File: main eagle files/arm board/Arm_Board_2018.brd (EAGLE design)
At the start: 193.8 x 104.4 mm, 152 parts, among them Q1 Q_IRF7437SMD, U1 TIVA-1294, U4 ACS722, U5 ACS722, U6 ACS722, U7 ACS722, U8 ACS722, U9 ACS722

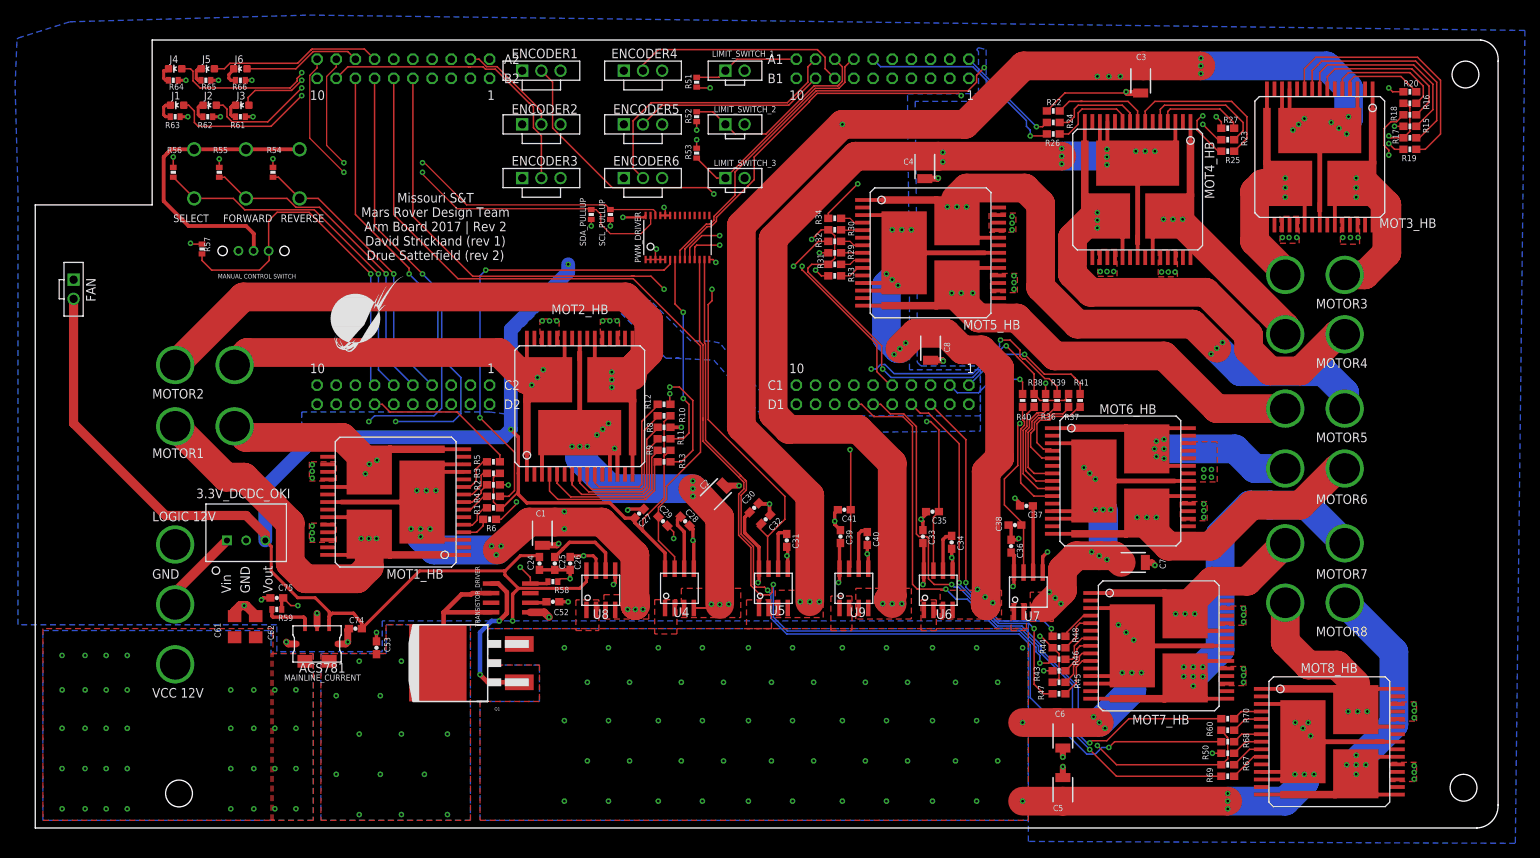
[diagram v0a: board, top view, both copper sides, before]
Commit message: added more polygons
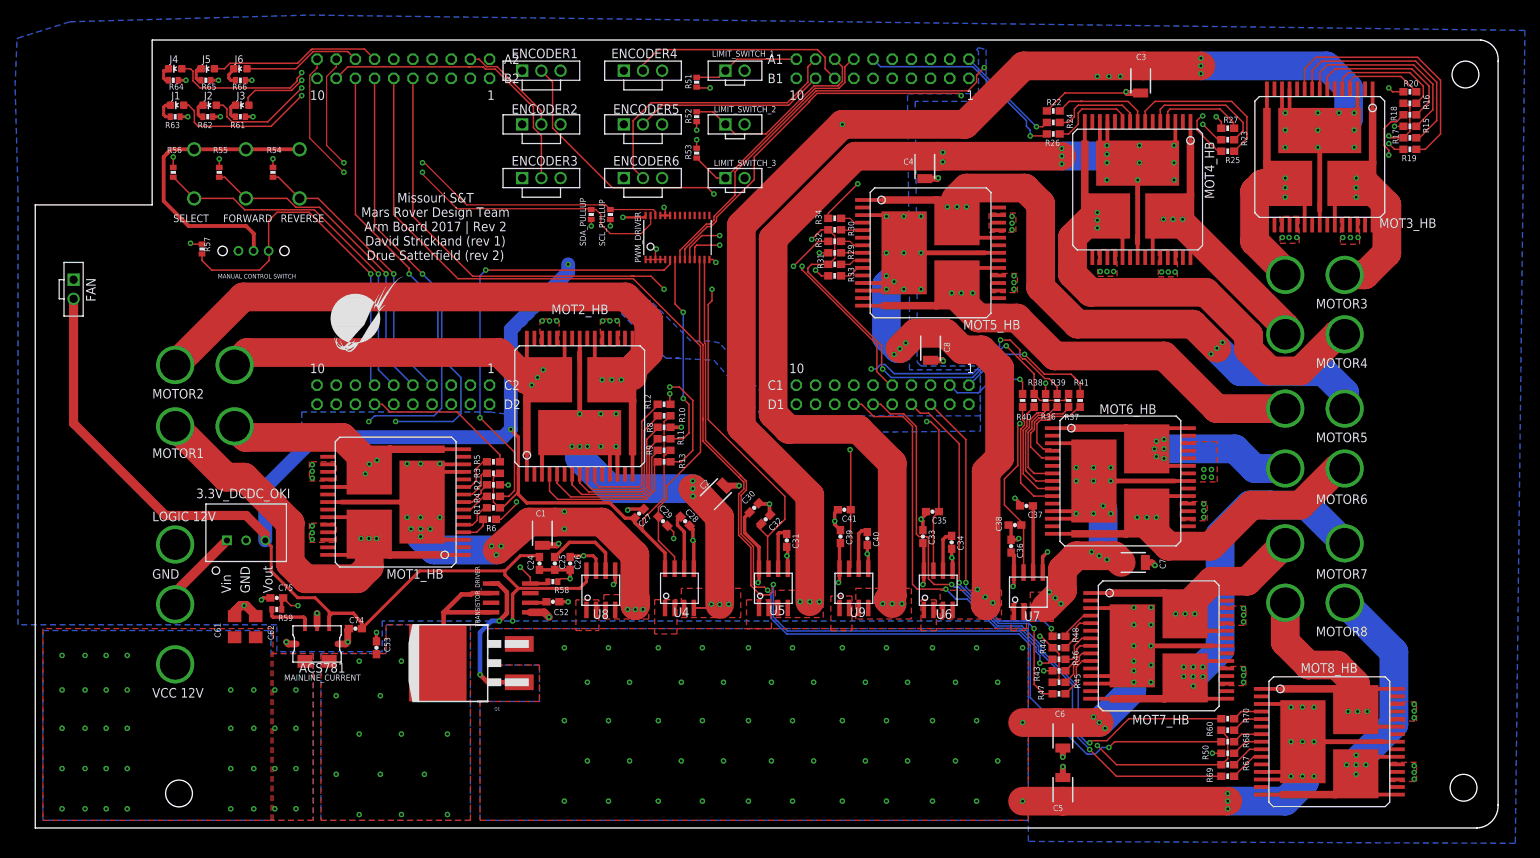
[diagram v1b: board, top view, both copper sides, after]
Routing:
- net MOTOR4_POWER: track 296.1 -> 308.0 mm, vias 14 -> 18
- net MOTOR3_POWER: track 374.3 -> 385.0 mm, vias 17 -> 20
- net MOTOR6_POWER: track 96.2 -> 89.4 mm, vias 12 -> 15
- net MOTOR2_POWER: track 135.4 -> 139.5 mm, vias 13 -> 14
- net MOTOR5_POWER: track 180.4 -> 177.2 mm, vias 12 -> 17
- net MOTOR1_POWER: track 146.1 -> 148.6 mm, vias 15 -> 18
- net 12VMOTOR_POWER: track 242.6 -> 244.8 mm, vias 72 -> 79
- net MOTOR2_2: track 182.7 -> 183.2 mm
- added copper zone on layer 2, net MOTOR1_POWER
- added copper zone on layer 2, net MOTOR2_POWER
- added copper zone on layer 2, net MOTOR3_POWER
- added copper zone on layer 2, net MOTOR4_POWER
- added copper zone on layer 2, net MOTOR5_POWER
- added copper zone on layer 2, net MOTOR6_POWER
